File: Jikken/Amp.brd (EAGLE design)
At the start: 100 x 80 mm, 17 parts, among them IC1 LF356N, U1 INPUT, U2 OUTPUT

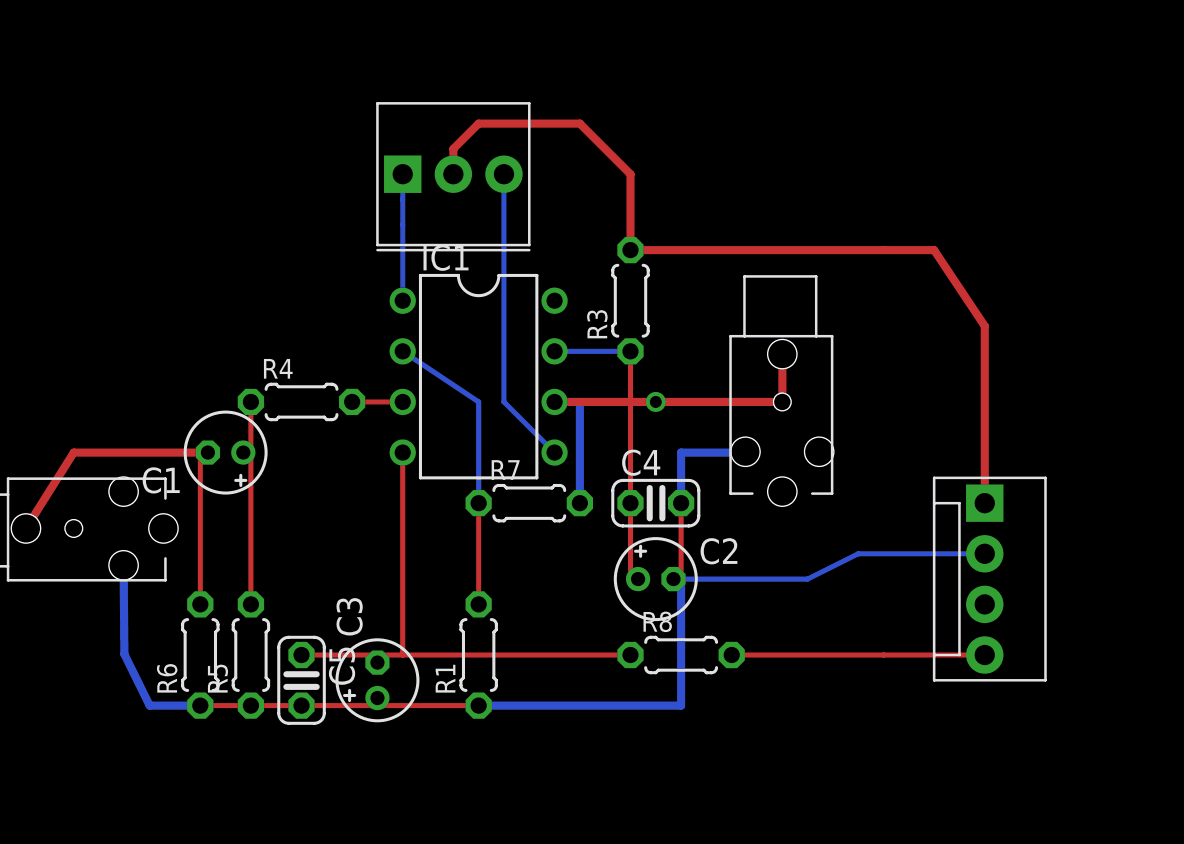
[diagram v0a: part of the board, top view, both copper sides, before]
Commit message: jikken
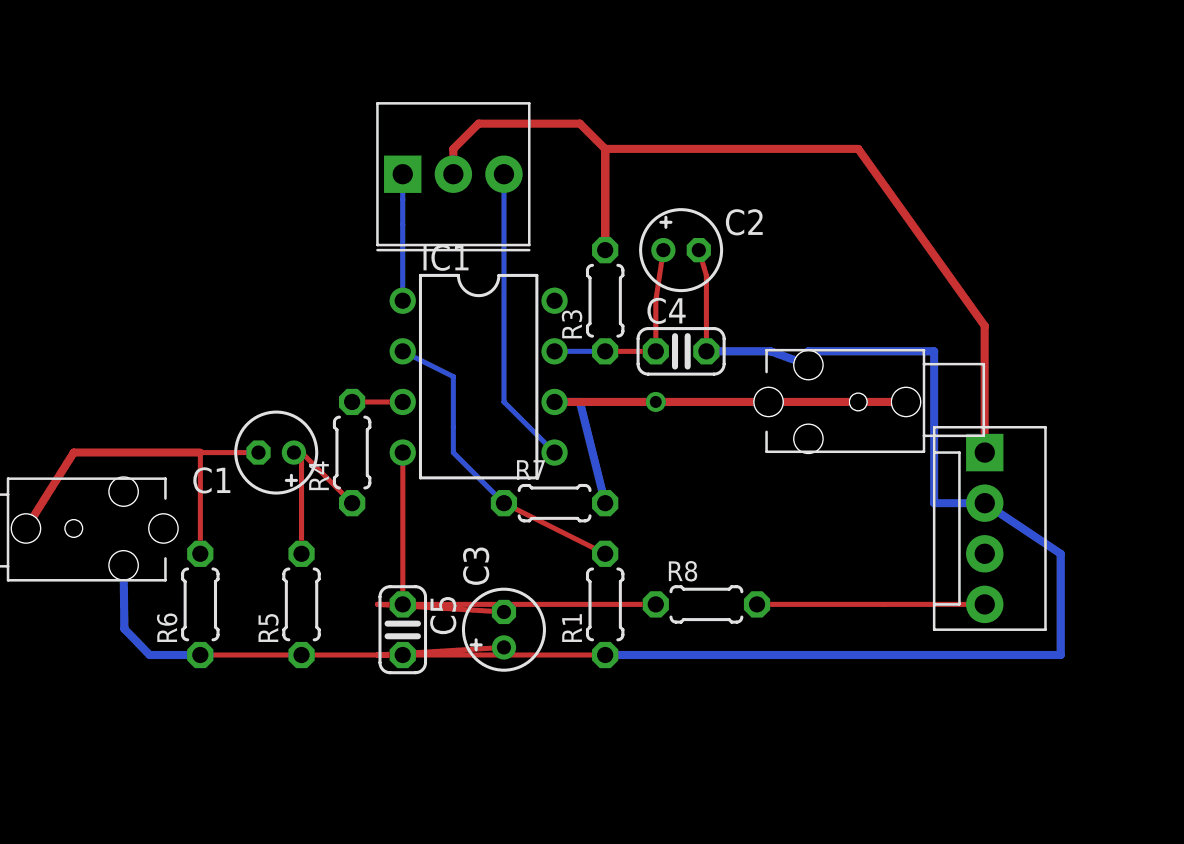
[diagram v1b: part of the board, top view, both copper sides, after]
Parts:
- moved C2 16.6 mm to (49.5, 59.7)
- moved C4 7.73 mm to (49.5, 54.6)
- moved C3 6.84 mm to (40.6, 40.6)
- moved R1 6.84 mm to (45.7, 41.9)
- moved C5 5.68 mm to (35.6, 40.6)
- moved U2 3.81 mm to (58.4, 52.1), turned to 180 degrees
- moved R4 3.59 mm to (33.0, 49.5), turned to 90 degrees
- moved R5 3.59 mm to (30.5, 41.9)
- moved R8 2.84 mm to (50.8, 41.9)
- moved C1 2.54 mm to (29.2, 49.5)
- moved JP1 2.54 mm to (64.8, 49.5)
- moved R6 2.54 mm to (25.4, 41.9)
- moved R3 1.27 mm to (45.7, 57.1)
- moved R7 1.27 mm to (43.2, 47.0)
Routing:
- net GND: track 66.7 -> 96.8 mm
- net VCC: track 44.3 -> 50.1 mm
- net N$9: track 15.6 -> 10.2 mm
- net N$7: track 20.2 -> 24.1 mm
- net N$5: track 27.1 -> 29.2 mm
- net N$2: track 10.9 -> 9.43 mm
- net -15V: track 12.7 -> 11.4 mm
- net N$4: track 14.7 -> 15.9 mm

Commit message: Amp
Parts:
- C1: value (none) -> 10u
- R7: value 200k -> 220k
- U$1: device SparkFun:3362U -> My Library:3362U
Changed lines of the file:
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@@
 <layer number="106" name="bPlate" color="7" fill="1" visible="no" active="yes"/>
 <layer number="107" name="Crop" color="7" fill="1" visible="no" active="yes"/>
+<layer number="108" name="fp8" color="7" fill="1" visible="no" active="yes"/>
+<layer number="109" name="fp9" color="7" fill="1" visible="no" active="yes"/>
+<layer number="110" name="fp0" color="7" fill="1" visible="no" active="yes"/>
 <layer number="116" name="Patch_BOT" color="9" fill="4" visible="no" active="yes"/>
 <layer number="121" name="_tsilk" color="7" fill="1" visible="no" active="yes"/>
 <layer number="122" name="_bsilk" color="7" fill="1" visible="no" active="yes"/>
+<layer number="123" name="tTestmark" color="7" fill="1" visible="no" active="yes"/>
+<layer number="124" name="bTestmark" color="7" fill="1" visible="no" active="yes"/>
 <layer number="125" name="_tNames" color="7" fill="1" visible="no" active="yes"/>
+<layer number="131" name="tAdjust" color="7" fill="1" visible="no" active="yes"/>
+<layer number="132" name="bAdjust" color="7" fill="1" visible="no" active="yes"/>
 <layer number="144" name="Drill_legend" color="7" fill="1" visible="no" active="yes"/>
 <layer number="151" name="HeatSink" color="7" fill="1" visible="no" active="yes"/>
+<layer number="199" name="Contour" color="7" fill="1" visible="yes" active="yes"/>
 <layer number="200" name="200bmp" color="1" fill="10" visible="no" active="yes"/>
 <layer number="201" name="201bmp" color="2" fill="10" visible="no" active="yes"/>
@@
 <element name="R6" library="rcl" package="0204/5" value="2k2" x="25.4" y="41.91" rot="R90"/>
 <element name="R8" library="rcl" package="0204/5" value="10" x="50.8" y="41.91"/>
-<element name="C1" library="rcl" package="E1,8-4" value="" x="29.21" y="49.53" rot="R180"/>
+<element name="C1" library="rcl" package="E1,8-4" value="10u" x="29.21" y="49.53" rot="R180"/>
 <element name="C2" library="rcl" package="E1,8-4" value="10u" x="49.53" y="59.69"/>
 <element name="C3" library="rcl" package="E1,8-4" value="10u" x="40.64" y="40.64" rot="R90"/>
 <element name="C4" library="rcl" package="C025-024X044" value="0.1u" x="49.53" y="54.61"/>
 <element name="C5" library="rcl" package="C025-024X044" value="0.1u" x="35.56" y="40.64" rot="R270"/>
-<element name="U$1" library="SparkFun" package="3362U" value="20k" x="35.56" y="60.96"/>
-<element name="R7" library="rcl" package="0204/5" value="200k" x="43.18" y="46.99"/>
+<element name="U$1" library="My Library" package="3362U" value="20k" x="35.56" y="60.96"/>
+<element name="R7" library="rcl" package="0204/5" value="220k" x="43.18" y="46.99"/>
 <element name="U1" library="SparkFun" package="STEREOJACK2.5MM_SPECIAL_HOLES-ONLY" value="INPUT" x="19.05" y="45.72"/>
 <element name="JP1" library="SparkFun" package="MOLEX-1X4" value="POWER" x="64.77" y="49.53" rot="R270"/>
